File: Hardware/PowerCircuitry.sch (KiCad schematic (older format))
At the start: 37 parts, among them J4 Conn_01x02_Male, Q5 MTP3055VL, Q6 MTP3055VL, Q7 2N2219, SW3 SW_SPST, U4 MAX40200AUK

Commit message: Some connections
I hope this is ok
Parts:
- Q5, Q6: symbol MTP3055VL:MTP3055VL -> VLAD-rescue:MTP3055VL-MTP3055VL
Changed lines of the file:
@@
 EESchema Schematic File Version 4
-LIBS:VLAD-cache
 EELAYER 30 0
 EELAYER END
@@
 	2950 6500 3200 6500
 $Comp
-L MTP3055VL:MTP3055VL Q5
+L VLAD-rescue:MTP3055VL-MTP3055VL Q5
 U 1 1 60AA2630
 P 1400 1500
@@
 Source1
 $Comp
-L MTP3055VL:MTP3055VL Q6
+L VLAD-rescue:MTP3055VL-MTP3055VL Q6
 U 1 1 60AC0CD1
 P 1400 2250

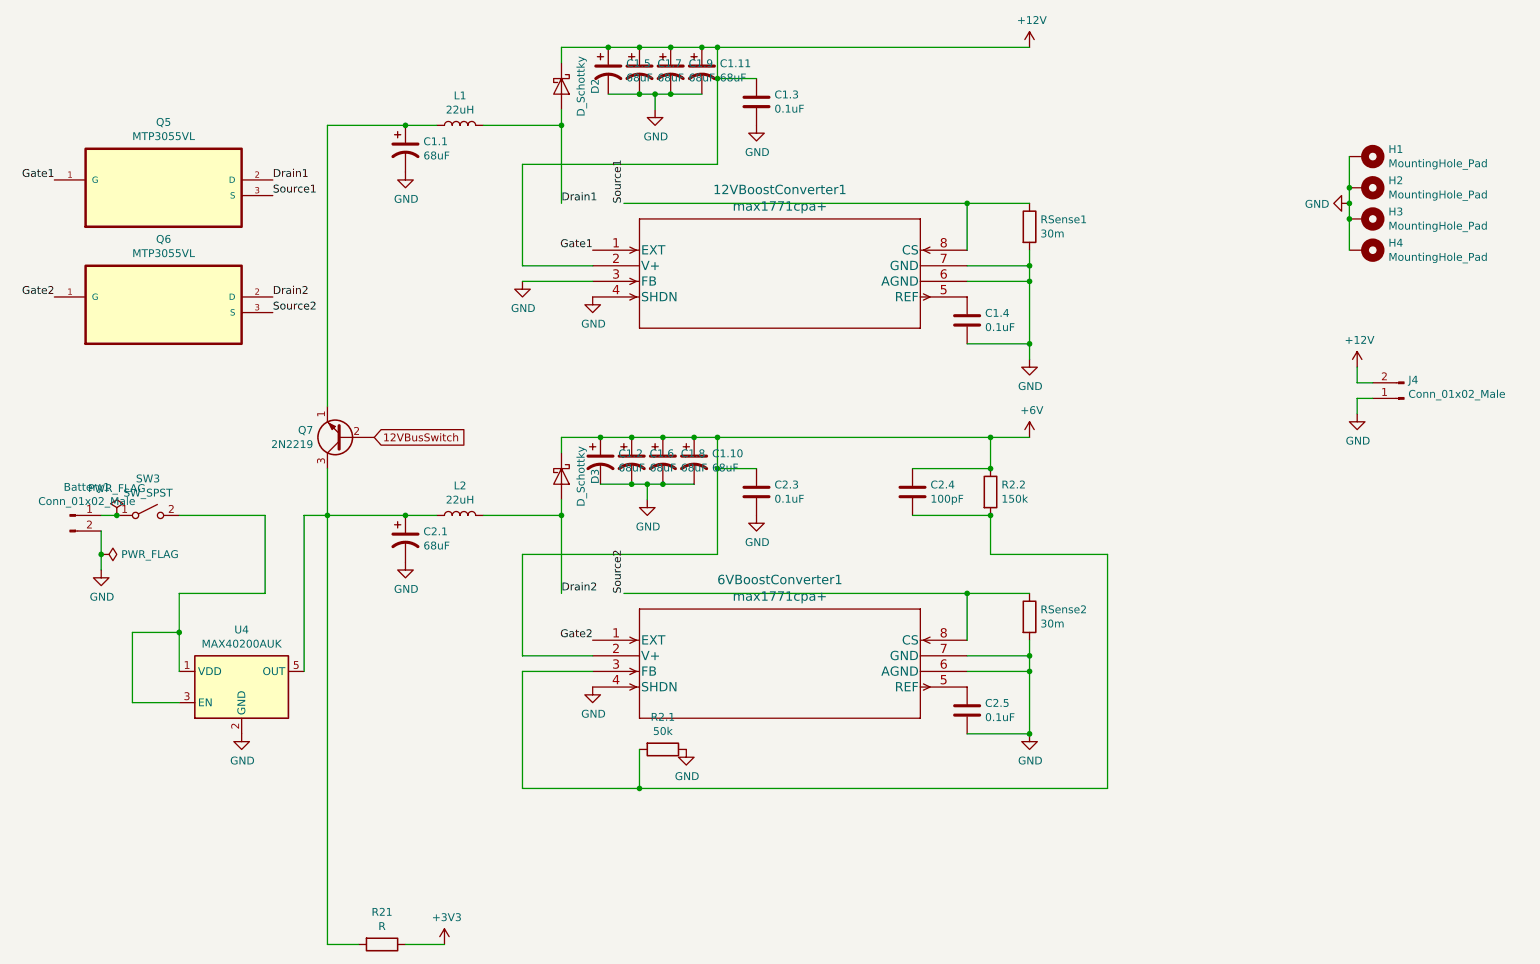
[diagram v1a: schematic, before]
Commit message: Added lots of things - needs some redoing
Fun, but ffs could have been easier
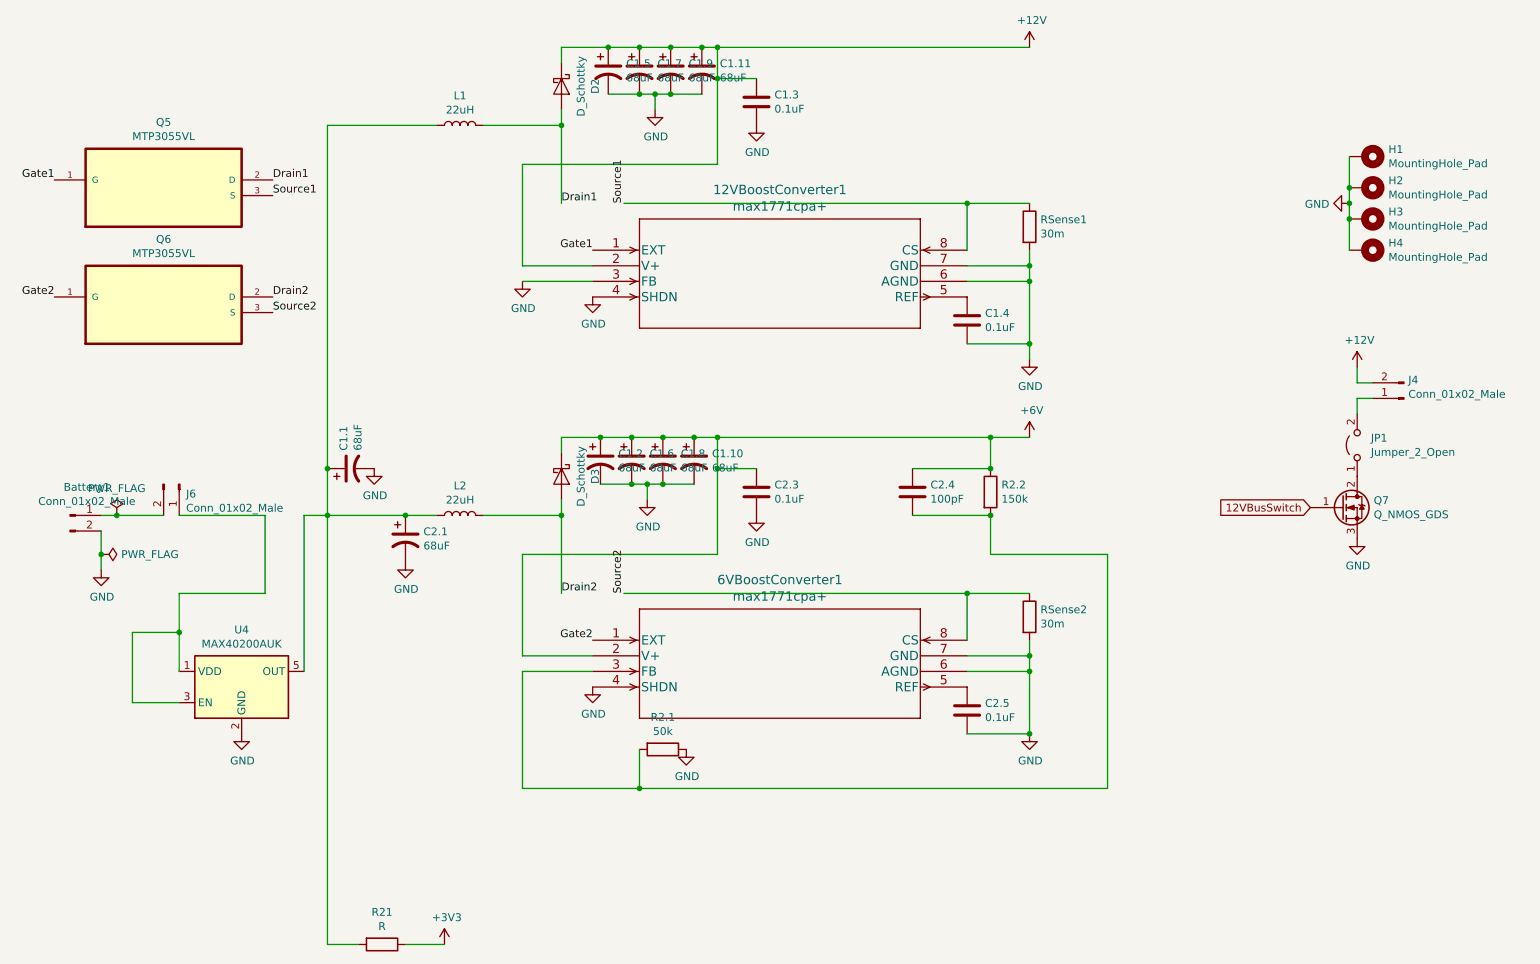
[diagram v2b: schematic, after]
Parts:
- removed Q7: 2N2219, Package_TO_SOT_THT:TO-92_Inline, symbol Transistor_BJT:2N2219
- removed SW3: SW_SPST, Button_Switch_THT:SW_DIP_SPSTx01_Slide_9.78x4.72mm_W7.62mm_P2.54mm, symbol Switch:SW_SPST
- added J6: Conn_01x02_Male, Connector_PinHeader_2.54mm:PinHeader_1x02_P2.54mm_Vertical, symbol Connector:Conn_01x02_Male
- added JP1: Jumper_2_Open, Connector_PinHeader_2.54mm:PinHeader_1x02_P2.54mm_Vertical, symbol Jumper:Jumper_2_Open
- added Q7: Q_NMOS_GDS, Package_TO_SOT_SMD:SOT-23, symbol Device:Q_NMOS_GDS
- Q5, Q6: footprint Package_TO_SOT_THT:TO-220-3_Vertical -> Package_TO_SOT_SMD:SOT-23
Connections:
- net 12VBusSwitch: now also Q7.1 (G)
- net GND: now also Q7.3 (S); no longer J4.1 (Pin_1)
- net at C1.1.1, L1.1: now also C2.1.1, L2.1, R21.2, U4.5 (OUT)
- net at Battery1.1 (Pin_1): now also J6.2 (Pin_2)
- net at U4.1 (VDD), U4.3 (EN): now also J6.1 (Pin_1)
- new net: J4.1 (Pin_1), JP1.2 (B)
- new net: JP1.1 (A), Q7.2 (D)
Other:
- moved on the sheet: C1.1
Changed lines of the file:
@@
 EESchema Schematic File Version 4
+LIBS:VLAD-cache
 EELAYER 30 0
 EELAYER END
@@
 	0    -1   -1   0
 $EndComp
-Wire Wire Line
-	2950 1250 3150 1250
 $Comp
 L power:GND #PWR036
 U 1 1 607A1CEB
-P 2950 1550
-F 0 "#PWR036" H 2950 1300 50  0001 C CNN
-F 1 "GND" H 2955 1377 50  0000 C CNN
-F 2 "" H 2950 1550 50  0001 C CNN
-F 3 "" H 2950 1550 50  0001 C CNN
-	1    2950 1550
+P 2750 3450
+F 0 "#PWR036" H 2750 3200 50  0001 C CNN
+F 1 "GND" H 2755 3277 50  0000 C CNN
+F 2 "" H 2750 3450 50  0001 C CNN
+F 3 "" H 2750 3450 50  0001 C CNN
+	1    2750 3450
 	1    0    0    -1
 $EndComp
@@
 L Device:CP1 C1.1
 U 1 1 607A0DAB
-P 2950 1400
-F 0 "C1.1" H 3065 1446 50  0000 L CNN
-F 1 "68uF" H 3065 1355 50  0000 L CNN
-F 2 "Capacitor_THT:CP_Radial_D6.3mm_P2.50mm" H 2950 1400 50  0001 C CNN
-F 3 "~" H 2950 1400 50  0001 C CNN
-	1    2950 1400
-	1    0    0    -1
+P 2600 3450
+F 0 "C1.1" H 2715 3496 50  0000 L CNN
+F 1 "68uF" H 2715 3405 50  0000 L CNN
+F 2 "Capacitor_THT:CP_Radial_D6.3mm_P2.50mm" H 2600 3450 50  0001 C CNN
+F 3 "~" H 2600 3450 50  0001 C CNN
+	1    2600 3450
+	0    -1   -1   0
 $EndComp
 $Comp
@@
 L power:GND #PWR055
 U 1 1 609E5451
-P 9050 3100
-F 0 "#PWR055" H 9050 2850 50  0001 C CNN
-F 1 "GND" H 9055 2927 50  0000 C CNN
-F 2 "" H 9050 3100 50  0001 C CNN
-F 3 "" H 9050 3100 50  0001 C CNN
-	1    9050 3100
+P 9050 3900
+F 0 "#PWR055" H 9050 3650 50  0001 C CNN
+F 1 "GND" H 9055 3727 50  0000 C CNN
+F 2 "" H 9050 3900 50  0001 C CNN
+F 3 "" H 9050 3900 50  0001 C CNN
+	1    9050 3900
 	1    0    0    -1
 $EndComp
 Connection ~ 1100 3750
-$Comp
-L Switch:SW_SPST SW3
-U 1 1 608DCB23
-P 1300 3750
-F 0 "SW3" H 1300 3985 50  0000 C CNN
-F 1 "SW_SPST" H 1300 3894 50  0000 C CNN
-F 2 "Button_Switch_THT:SW_DIP_SPSTx01_Slide_9.78x4.72mm_W7.62mm_P2.54mm" H 1300 3750 50  0001 C CNN
-F 3 "~" H 1300 3750 50  0001 C CNN
-	1    1300 3750
-	1    0    0    -1
-$EndComp
 Wire Wire Line
 	2050 3750 2050 4250
@@
 Wire Wire Line
 	4500 3550 4600 3550
-$Comp
-L Transistor_BJT:2N2219 Q7
-U 1 1 60A91052
-P 2550 3250
-F 0 "Q7" H 2741 3204 50  0000 L CNN
-F 1 "2N2219" H 2741 3295 50  0000 L CNN
-F 2 "Package_TO_SOT_THT:TO-92_Inline" H 2750 3175 50  0001 L CIN
-F 3 "http://www.onsemi.com/pub_link/Collateral/2N2219-D.PDF" H 2550 3250 50  0001 L CNN
-	1    2550 3250
-	-1   0    0    1
-$EndComp
 Wire Wire Line
 	2450 3450 2450 3750
-Wire Wire Line
-	2450 3050 2450 1250
-Wire Wire Line
-	2450 1250 2950 1250
-Connection ~ 2950 1250
-Text GLabel 2750 3250 2    50   Input ~ 0
-12VBusSwitch
 $Comp
 L Device:R R21
@@
 F 0 "Q5" H 1400 1770 50  0000 C CNN
 F 1 "MTP3055VL" H 1400 1679 50  0000 C CNN
-F 2 "Package_TO_SOT_THT:TO-220-3_Vertical" H 1400 1500 50  0001 L BNN
+F 2 "Package_TO_SOT_SMD:SOT-23" H 1400 1500 50  0001 L BNN
 F 3 "" H 1400 1500 50  0001 L BNN
 F 4 "MTP3055VL" H 1400 1500 50  0001 L BNN "MPN"
@@
 F 0 "Q6" H 1400 2520 50  0000 C CNN
 F 1 "MTP3055VL" H 1400 2429 50  0000 C CNN
-F 2 "Package_TO_SOT_THT:TO-220-3_Vertical" H 1400 2250 50  0001 L BNN
+F 2 "Package_TO_SOT_SMD:SOT-23" H 1400 2250 50  0001 L BNN
 F 3 "" H 1400 2250 50  0001 L BNN
 F 4 "MTP3055VL" H 1400 2250 50  0001 L BNN "MPN"
@@
 Text Label 4350 4250 1    50   ~ 0
 Source2
+$Comp
+L Connector:Conn_01x02_Male J6
+U 1 1 60AE4D44
+P 1500 3550
+F 0 "J6" V 1562 3594 50  0000 L CNN
+F 1 "Conn_01x02_Male" V 1653 3594 50  0000 L CNN
+F 2 "Connector_PinHeader_2.54mm:PinHeader_1x02_P2.54mm_Vertical" H 1500 3550 50  0001 C CNN
+F 3 "~" H 1500 3550 50  0001 C CNN
+	1    1500 3550
+	0    1    1    0
+$EndComp
+Wire Wire Line
+	1100 3750 1400 3750
+Connection ~ 2450 3450
+Wire Wire Line
+	2450 1250 3150 1250
+Wire Wire Line
+	2450 1250 2450 3450
+$Comp
+L Device:Q_NMOS_GDS Q7
+U 1 1 60B1F303
+P 8950 3700
+F 0 "Q7" H 9156 3746 50  0000 L CNN
+F 1 "Q_NMOS_GDS" H 9156 3655 50  0000 L CNN
+F 2 "Package_TO_SOT_SMD:SOT-23" H 9150 3800 50  0001 C CNN
+F 3 "~" H 8950 3700 50  0001 C CNN
+	1    8950 3700
+	1    0    0    -1
+$EndComp
+Text GLabel 8750 3700 0    50   Input ~ 0
+12VBusSwitch
+$Comp
+L Jumper:Jumper_2_Open JP1
+U 1 1 60B321AD
+P 9050 3300
+F 0 "JP1" V 9096 3212 50  0000 R CNN
+F 1 "Jumper_2_Open" V 9005 3212 50  0000 R CNN
+F 2 "Connector_PinHeader_2.54mm:PinHeader_1x02_P2.54mm_Vertical" H 9050 3300 50  0001 C CNN
+F 3 "~" H 9050 3300 50  0001 C CNN
+	1    9050 3300
+	0    -1   -1   0
+$EndComp
 $EndSCHEMATC
